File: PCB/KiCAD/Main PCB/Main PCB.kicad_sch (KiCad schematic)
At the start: 81 parts, among them J1 Conn_01x04, J2 Conn_02x03_Odd_Even, J3 Conn_02x03_Odd_Even, J4 Conn_01x08, J5 Conn_01x02, J6 Conn_01x02, Q1 BSS138, Q2 BSS138, U1 Teensy4.0, U2 MIC5219-3.3YM5

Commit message: Changes to the main PCB
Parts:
- removed D1: RED_LED, LED_SMD:LED_0805_2012Metric_Pad1.15x1.40mm_HandSolder, symbol Device:LED
- removed D10, D11, D12, D13, D14, D15, D16, D17, D18, D19, D20, D21, D22, D7, D8, D9: BALL_DIR_LED, LED_SMD:LED_0805_2012Metric_Pad1.15x1.40mm_HandSolder, symbol Device:LED
- removed D2: GREEN_LED, LED_SMD:LED_0805_2012Metric_Pad1.15x1.40mm_HandSolder, symbol Device:LED
- removed D3, D4, D5, D6: LED, LED_SMD:LED_0805_2012Metric_Pad1.15x1.40mm_HandSolder, symbol Device:LED
- removed J1: Conn_01x04, Connector_JST:JST_PH_B4B-PH-K_1x04_P2.00mm_Vertical, symbol Connector_Generic:Conn_01x04
- removed J2, J3: Conn_02x03_Odd_Even, Connector_IDC:IDC-Header_2x03_P2.54mm_Vertical_SMD, symbol Connector_Generic:Conn_02x03_Odd_Even
- removed J4: Conn_01x08, Connector_JST:JST_PH_B8B-PH-K_1x08_P2.00mm_Vertical, symbol Connector_Generic:Conn_01x08
- removed R15, R16, R17, R18: 1k, Resistor_SMD:R_0805_2012Metric_Pad1.20x1.40mm_HandSolder, symbol Device:R
- removed R21, R22, R23, R24, R25, R26, R27, R28, R29, R30, R31, R32, R33, R34, R35, R36: 130, Resistor_SMD:R_0805_2012Metric_Pad1.20x1.40mm_HandSolder, symbol Device:R
- removed R4, R5: 330, Resistor_SMD:R_0805_2012Metric_Pad1.20x1.40mm_HandSolder, symbol Device:R
- removed S4, S5, S6: MSLPT5252BG4MTR, MSLPT5252BG4MTR:MSLPT5252BG4MTR, symbol MSLPT5252BG4MTR:MSLPT5252BG4MTR
- removed XBEE1, XBEE2: Conn_01x10, Connector_PinSocket_2.00mm:PinSocket_1x10_P2.00mm_Vertical, symbol Connector_Generic:Conn_01x10
- added F1: Fuse, Fuse:Fuseholder_Blade_Mini_Keystone_3568, symbol Device:Fuse
- added J1: Conn_01x02, Connector_AMASS:AMASS_XT60-M_1x02_P7.20mm_Vertical, symbol Connector_Generic:Conn_01x02
- added J5: Conn_01x02, Connector_JST:JST_PH_B2B-PH-K_1x02_P2.00mm_Vertical, symbol Connector_Generic:Conn_01x02
- added J6, J7: Conn_01x04, Connector_JST:JST_PH_B4B-PH-K_1x04_P2.00mm_Vertical, symbol Connector_Generic:Conn_01x04
- added S2: 1101M2S3CGE2, 1101M2S3CGE2:1101M2S3CGE2, symbol 1101M2S3CGE2:1101M2S3CGE2
- added U1: ~, Pololu:D36V28F5, symbol Pololu:D36V28F5
- added U2: Teensy4.1, Teensy:Teensy41, symbol teensy:Teensy4.1
- renumbered C1 to C24, C2 to C25, C3 to C26, J5 to J2, J6 to J3, Q2 to Q1, Q1 to Q2, R3 to R1, R20 to R10, R2 to R11, R7 to R12, R1 to R13, R6 to R14, R8 to R2, R11 to R3, R12 to R4, R13 to R5, R14 to R6, R9 to R7, R10 to R8, R19 to R9, S2 to S3, S3 to S4, U1 to U3, U2 to U8
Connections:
- net +3V3_XBEE is gone; now on net +3V3: C25.1, C26.1, U8.5 (OUT)
- net Earth is gone; now on net GND: J2.2 (Pin_2), R7.2, R8.2, R9.2
- net +3V3: no longer S3.2, S4.2, U3.31 (3V3)
- net +5V: now also U1.6 (OUT), U2.48 (VIN)
- net 3V3_SCL: now also U2.41 (19_A5_SCL)
- net 3V3_SDA: now also U2.40 (18_A4_SDA)
- net CALIBRATE_BUTTON: now also U2.13 (11_MOSI_CTX1); no longer U3.13 (11_MOSI_CTX1)
- net CAMERA_RX: now also U2.9 (7_RX2_OUT1A); no longer U3.9 (7_RX2_OUT1A)
- net CAMERA_TX: now also U2.10 (8_TX2_IN1); no longer U3.10 (8_TX2_IN1)
- net COM_RX: now also U2.43 (21_A7_RX5_BCLK1); no longer U3.2 (0_RX1_CRX2_CS1)
- net COM_TX: now also U2.42 (20_A6_TX5_LRCLK1); no longer U3.3 (1_TX1_CTX2_MISO1)
- net GND: now also J1.1 (Pin_1), J5.2 (Pin_2), U1.4 (GND_1), U1.5 (GND_2), U2.1 (GND), U2.34 (GND), U2.47 (GND), U2.52 (GND)
- net IR_DIR_0: now also U2.4 (2_OUT2); no longer U3.14 (12_MISO_MQSL)
- net IR_DIR_112.5: now also U2.27 (35_TX8); no longer U3.37 (26_A12_MOSI1)
- net IR_DIR_135: now also U2.36 (14_A0_TX3_SPDIF_OUT); no longer U3.28 (21_A7_RX5_BCLK1)
- net IR_DIR_157.5: now also U2.28 (36_CS); no longer U3.38 (27_A13_SCK1)
- net IR_DIR_180: now also U2.6 (4_BCLK2); no longer U3.23 (16_A2_RX4_SCL1)
- net IR_DIR_202.5: now also U2.29 (37_CS); no longer U3.39 (28_RX7)
- net IR_DIR_22.5: now also U2.25 (33_MCLK2); no longer U3.35 (24_A10_TX6_SCL2)
- net IR_DIR_225: now also U2.37 (15_A1_RX3_SPDIF_IN); no longer U3.29 (22_A8_CTX1)
- net IR_DIR_247.5: now also U2.30 (38_CS1_IN1); no longer U3.40 (29_TX7)
- net IR_DIR_270: now also U2.7 (5_IN2); no longer U3.24 (17_A3_TX4_SDA1)
- net IR_DIR_292.5: now also U2.31 (39_MISO1_OUT1A); no longer U3.41 (30_CRX3)
- net IR_DIR_315: now also U2.38 (16_A2_RX4_SCL1); no longer U3.30 (23_A9_CRX1_MCLK1)
- net IR_DIR_337.5: now also U2.32 (40_A16); no longer U3.42 (31_CTX3)
- net IR_DIR_45: now also U2.14 (12_MISO_MQSL); no longer U3.27 (20_A6_TX5_LRCLK1)
- net IR_DIR_67.5: now also U2.26 (34_RX8); no longer U3.36 (25_A11_RX6_SDA2)
- net IR_DIR_90: now also U2.5 (3_LRCLK2); no longer U3.22 (15_A1_RX3_SPDIF_IN)
- net LG_RECEIVE: now also U3.22 (15_A1_RX3_SPDIF_IN); no longer U3.21 (14_A0_TX3_SPDIF_OUT)
- net START_BUTTON: now also U2.12 (10_CS_MQSR); no longer U3.12 (10_CS_MQSR)
- net at R3.2, S1.B3: now also U2.21 (29_TX7); no longer U3.6 (4_BCLK2)
- net at R4.2, S1.B4: now also U2.22 (30_CRX3); no longer U3.7 (5_IN2)
- net at R2.2, S1.B2: now also U2.20 (28_RX7); no longer U3.5 (3_LRCLK2)
- net at R6.2, S1.B6: now also U2.24 (32_OUT1B); no longer U3.43 (32_OUT1B)
- net at R1.2, S1.B1: now also U2.19 (27_A13_SCK1); no longer U3.4 (2_OUT2)
- net TSSP_2_A2: now reaches U3.44 (33_MCLK2)
- net at R5.2, S1.B5: now also U2.23 (31_CTX3); no longer U3.8 (6_OUT1D)
- net STATUS_GREEN renamed MOTOR_4_DIR
- net STATUS_RED renamed STATUS_RED_4_0
- new net: F1.1, J1.2 (Pin_2)
- new net: F1.2, S2.2 (COM)
- new net +12V: S2.3 (NO), U1.3 (IN)
- new net +3V3_4_0: J5.1 (Pin_1), U3.31 (3V3)
- new net +3V3_4_1: S3.2, S4.2, U2.46 (3V3)
- new net LED_1_A0: J6.2 (Pin_2), U3.13 (11_MOSI_CTX1)
- new net LED_1_A1: J6.3 (Pin_3), U3.14 (12_MISO_MQSL)
- new net LED_1_A2: J6.4 (Pin_4), U3.23 (16_A2_RX4_SCL1)
- new net LED_1_OUT: J6.1 (Pin_1), U3.12 (10_CS_MQSR)
- new net LED_2_A0: J7.2 (Pin_2), U3.27 (20_A6_TX5_LRCLK1)
- new net LED_2_A1: J7.3 (Pin_3), U3.28 (21_A7_RX5_BCLK1)
- new net LED_2_A2: J7.4 (Pin_4), U3.35 (24_A10_TX6_SCL2)
- new net LED_2_OUT: J7.1 (Pin_1), U3.24 (17_A3_TX4_SDA1)
- new net MOTOR_1_DIR: U3.5 (3_LRCLK2)
- new net MOTOR_1_SPEED: U3.4 (2_OUT2)
- new net MOTOR_2_DIR: U3.7 (5_IN2)
- new net MOTOR_2_SPEED: U3.6 (4_BCLK2)
- new net MOTOR_3_DIR: U3.9 (7_RX2_OUT1A)
- new net MOTOR_3_SPEED: U3.8 (6_OUT1D)
- new net MOTOR_4_SPEED: U3.10 (8_TX2_IN1)
- new net STATUS_GREEN_4_0: U3.21 (14_A0_TX3_SPDIF_OUT)
- new net STATUS_GREEN_4_1: U2.11 (9_OUT1C)
- new net STATUS_RED_4_1: U2.35 (13_SCK_LED)
- new net TEENSY_RX: U2.2 (0_RX1_CRX2_CS1), U3.3 (1_TX1_CTX2_MISO1)
- new net TEENSY_TX: U2.3 (1_TX1_CTX2_MISO1), U3.2 (0_RX1_CRX2_CS1)
- new net TSSP_1_A0: U3.39 (28_RX7)
- new net TSSP_1_A1: U3.40 (29_TX7)
- new net TSSP_1_A2: U3.41 (30_CRX3)
- new net TSSP_1_OUT: U3.29 (22_A8_CTX1)
- new net TSSP_2_A0: U3.42 (31_CTX3)
- new net TSSP_2_A1: U3.43 (32_OUT1B)
- new net TSSP_2_OUT: U3.30 (23_A9_CRX1_MCLK1)
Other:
- added sheet Communication (communication.kicad_sch)
- added sheet LED Indicators (led_indicators.kicad_sch)
- added sheet Motors (motors.kicad_sch)
- moved on the sheet: C24, C25, C26, CAM1, CAM2, J2, J3, Q1, Q2, R1, R10, R11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

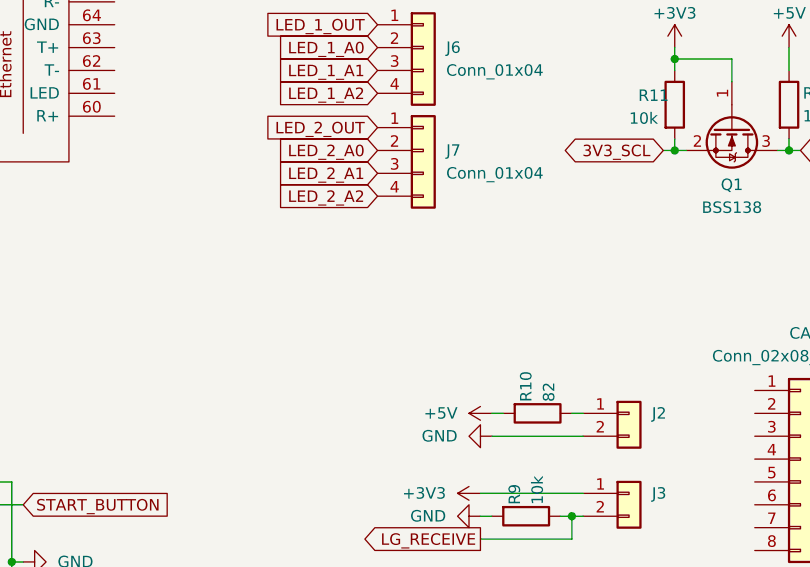
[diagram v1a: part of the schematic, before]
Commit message: Updated to main PCB
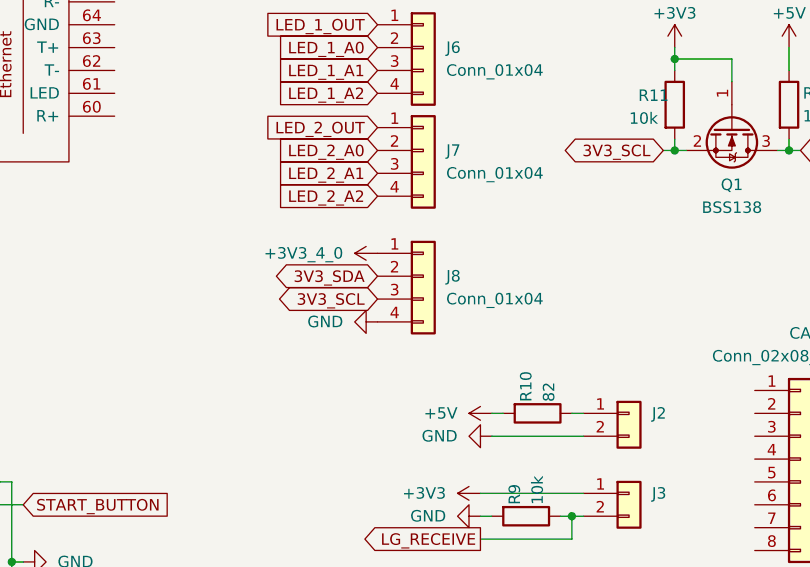
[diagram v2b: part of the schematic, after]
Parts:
- added J8: Conn_01x04, Connector_JST:JST_PH_B4B-PH-K_1x04_P2.00mm_Vertical, symbol Connector_Generic:Conn_01x04
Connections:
- net +3V3_4_0: now also J8.1 (Pin_1)
- net 3V3_SCL: now also J8.3 (Pin_3)
- net 3V3_SDA: now also J8.2 (Pin_2)
- net GND: now also J8.4 (Pin_4)
